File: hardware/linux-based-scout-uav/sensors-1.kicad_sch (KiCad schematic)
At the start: 1 part, among them U5 MPU-6050

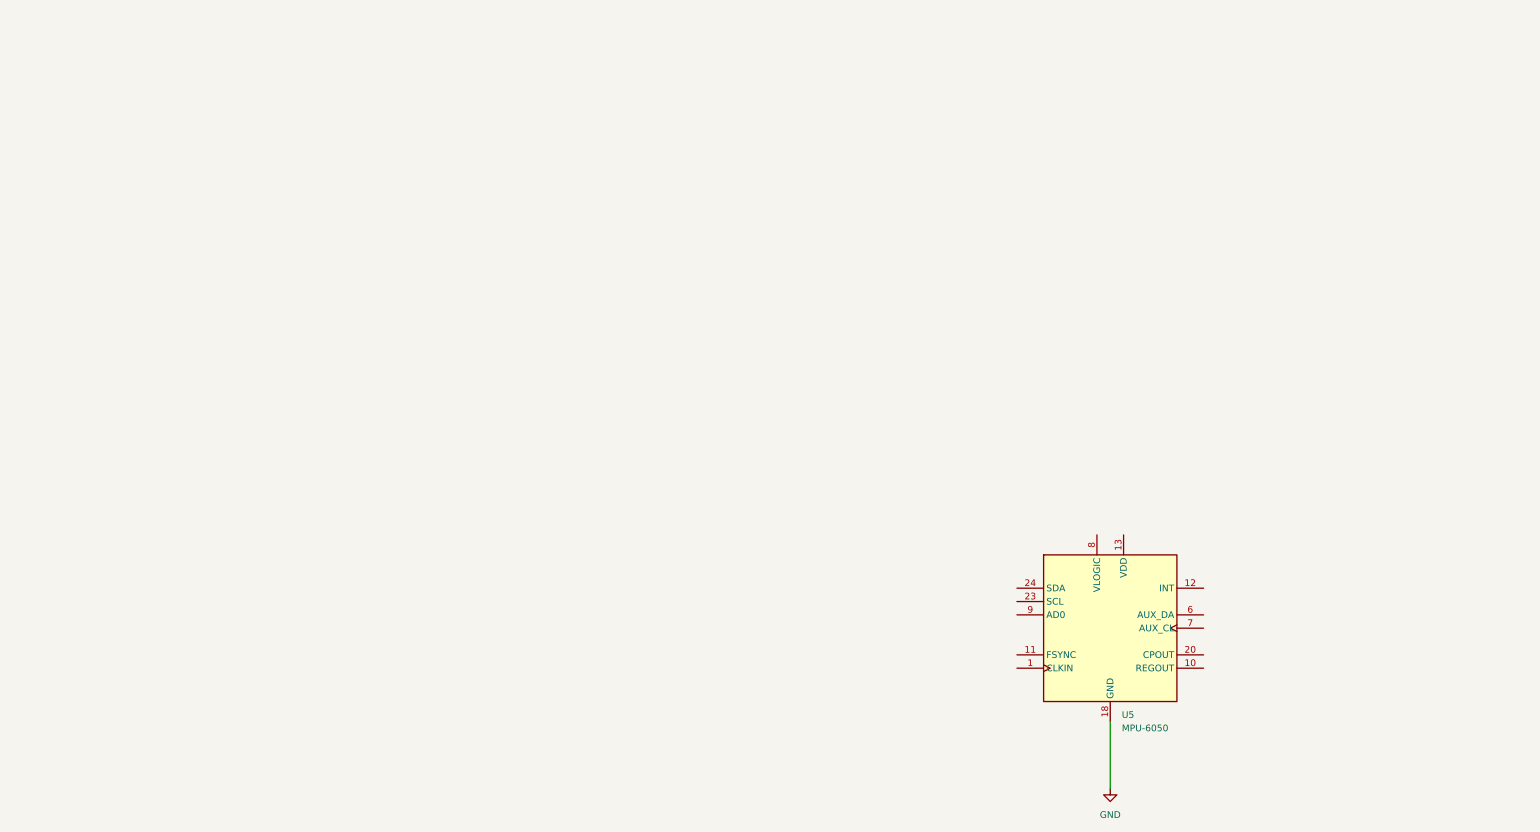
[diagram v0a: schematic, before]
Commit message: Schematic update
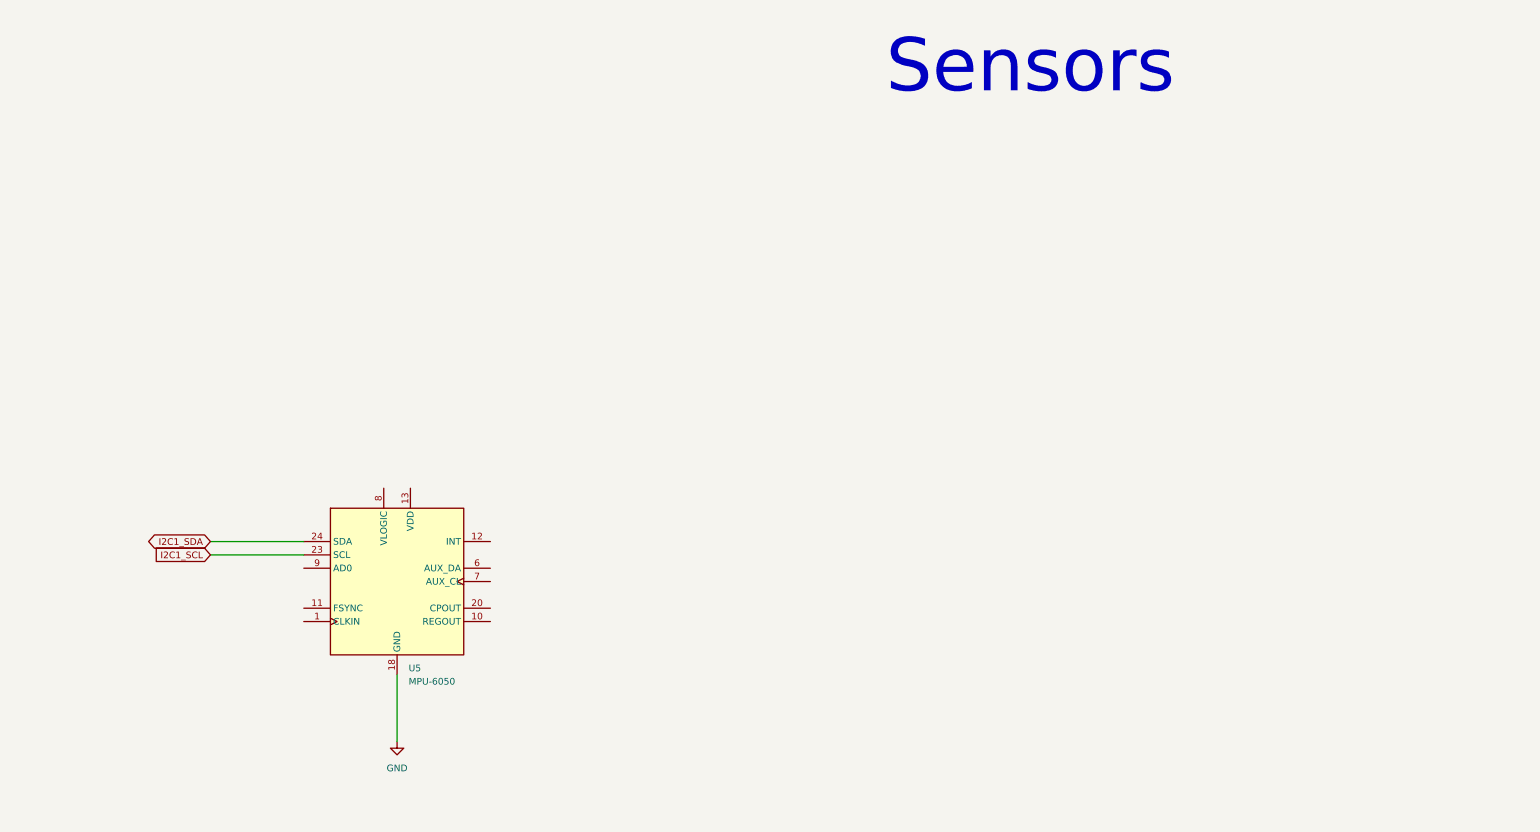
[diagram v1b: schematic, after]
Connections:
- net I2C1_SCL: now reaches U5.23 (SCL)
- net I2C1_SDA: now reaches U5.24 (SDA)
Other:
- note added: "Sensors"
- moved on the sheet: U5
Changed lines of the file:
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@@
 	(wire
 		(pts
-			(xy 228.6 157.48) (xy 228.6 170.18)
+			(xy 92.71 148.59) (xy 92.71 161.29)
 		)
 		(stroke
@@
 		)
 	)
+	(wire
+		(pts
+			(xy 57.15 123.19) (xy 74.93 123.19)
+		)
+		(stroke
+			(width 0)
+			(type default)
+		)
+	)
+	(wire
+		(pts
+			(xy 57.15 125.73) (xy 74.93 125.73)
+		)
+		(stroke
+			(width 0)
+			(type default)
+		)
+	)
+	(text "Sensors"
+		(exclude_from_sim no)
+		(at 213.36 32.766 0)
+		(effects
+			(font
+				(face "KiCad Font")
+				(size 10.16 10.16)
+			)
+		)
+	)
+	(global_label "I2C1_SDA"
+		(shape bidirectional)
+		(at 57.15 123.19 180)
+		(fields_autoplaced yes)
+		(effects
+			(font
+				(size 1.27 1.27)
+			)
+			(justify right)
+		)
+		(property "Intersheetrefs" "${INTERSHEET_REFS}"
+			(at 44.224 123.19 0)
+			(effects
+				(font
+					(size 1.27 1.27)
+				)
+				(justify right)
+				(hide yes)
+			)
+		)
+	)
+	(global_label "I2C1_SCL"
+		(shape input)
+		(at 57.15 125.73 180)
+		(fields_autoplaced yes)
+		(effects
+			(font
+				(size 1.27 1.27)
+			)
+			(justify right)
+		)
+		(property "Intersheetrefs" "${INTERSHEET_REFS}"
+			(at 45.3958 125.73 0)
+			(effects
+				(font
+					(size 1.27 1.27)
+				)
+				(justify right)
+				(hide yes)
+			)
+		)
+	)
 	(symbol
 		(lib_id "Sensor_Motion:MPU-6050")
-		(at 228.6 139.7 0)
+		(at 92.71 130.81 0)
 		(unit 1)
 		(exclude_from_sim no)
@@
 		(fields_autoplaced yes)
 		(property "Reference" "U5"
-			(at 230.7941 156.21 0)
+			(at 94.9041 147.32 0)
 			(effects
 				(font
@@
 		)
 		(property "Value" "MPU-6050"
-			(at 230.7941 158.75 0)
+			(at 94.9041 149.86 0)
 			(effects
 				(font
@@
 		)
 		(property "Footprint" "Sensor_Motion:InvenSense_QFN-24_4x4mm_P0.5mm"
-			(at 228.6 160.02 0)
+			(at 92.71 151.13 0)
 			(effects
 				(font
@@
 		)
 		(property "Datasheet" "https://invensense.tdk.com/wp-content/uploads/2015/02/MPU-6000-Datasheet1.pdf"
-			(at 228.6 143.51 0)
+			(at 92.71 134.62 0)
 			(effects
 				(font
@@
 		)
 		(property "Description" "InvenSense 6-Axis Motion Sensor, Gyroscope, Accelerometer, I2C"
-			(at 228.6 139.7 0)
+			(at 92.71 130.81 0)
 			(effects
 				(font
@@
 	(symbol
 		(lib_id "power:GND")
-		(at 228.6 170.18 0)
+		(at 92.71 161.29 0)
 		(unit 1)
 		(exclude_from_sim no)
@@
 		(fields_autoplaced yes)
 		(property "Reference" "#PWR017"
-			(at 228.6 176.53 0)
+			(at 92.71 167.64 0)
 			(effects
 				(font
@@
 		)
 		(property "Value" "GND"
-			(at 228.6 175.26 0)
+			(at 92.71 166.37 0)
 			(effects
 				(font
@@
 		)
 		(property "Footprint" ""
-			(at 228.6 170.18 0)
+			(at 92.71 161.29 0)
 			(effects
 				(font
@@
 		)
 		(property "Datasheet" ""
-			(at 228.6 170.18 0)
+			(at 92.71 161.29 0)
 			(effects
 				(font
@@
 		)
 		(property "Description" "Power symbol creates a global label with name \"GND\" , ground"
-			(at 228.6 170.18 0)
-			(effects
-				(font
+			(at 92.71 161.29 0)
+			(effects
+				(font

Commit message: Schematic update
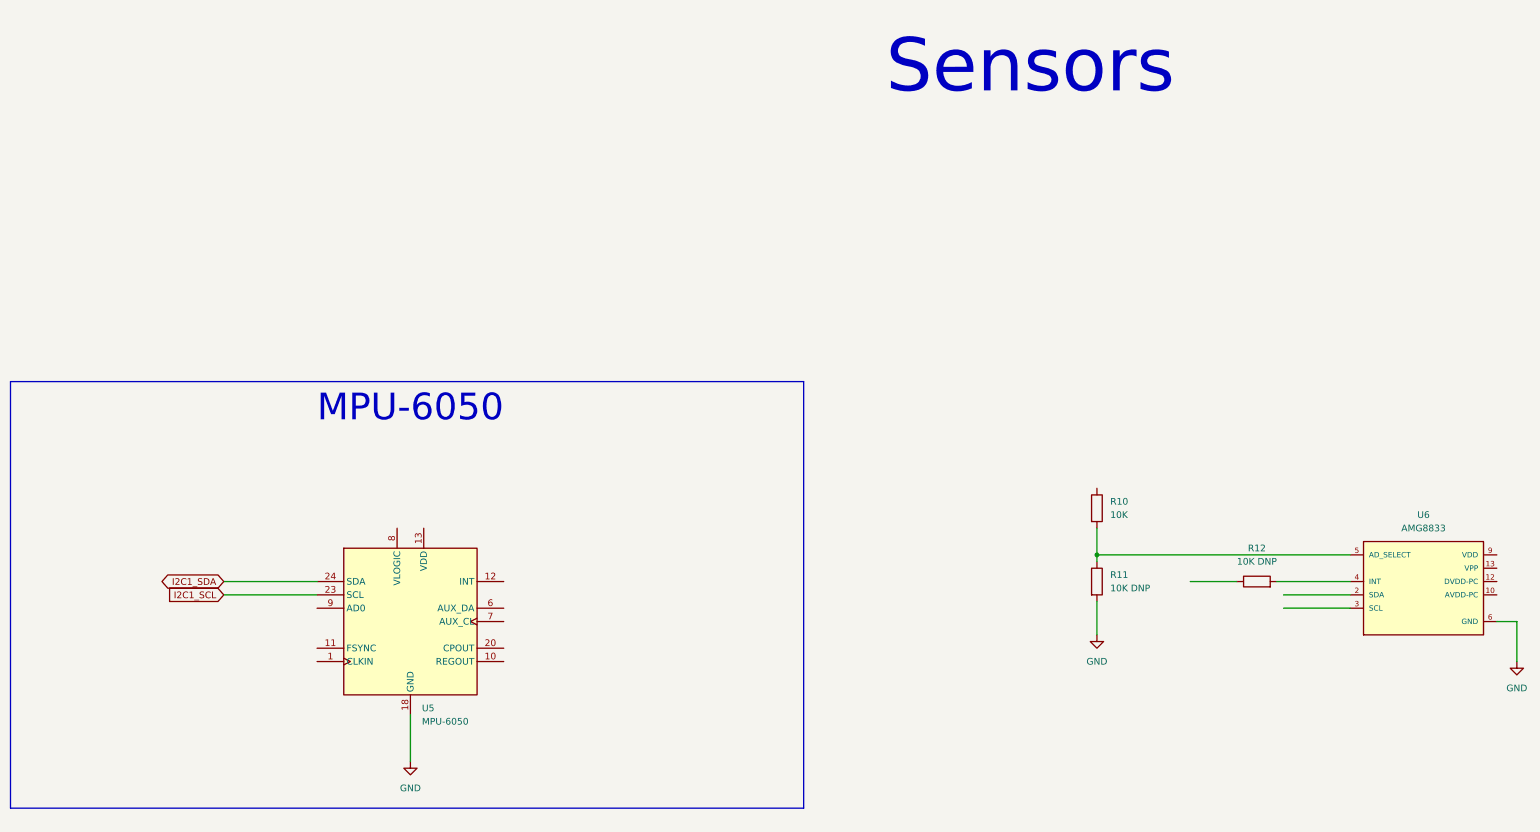
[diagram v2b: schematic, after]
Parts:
- added R10: 10K, Resistor_SMD:R_0402_1005Metric, symbol Device:R
- added R11, R12: 10K DNP, Resistor_SMD:R_0402_1005Metric, symbol Device:R
- added U6: AMG8833, AMG8833:XDCR_AMG8833, symbol AMG8833:AMG8833
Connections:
- net GND: now also R11.2, U6.6 (GND)
- new net: R12.2, U6.4 (INT)
- new net: R10.2, R11.1, U6.5 (AD_SELECT)
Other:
- note added: "MPU-6050"
- moved on the sheet: U5
